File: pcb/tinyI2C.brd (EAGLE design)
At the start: 83.2 x 83.2 mm, 29 parts, among them IC1 IC_TTL_74_125, IC2 TPS73618(0.4A), U1 LPC824M201JHI33, X1 TSW-112-02-S-S, X2 TSW-106-02-S-S-RA, X3 TSW-112-02-S-S, X4 TSW-102-02-S-S, X5 TSW-102-02-S-S

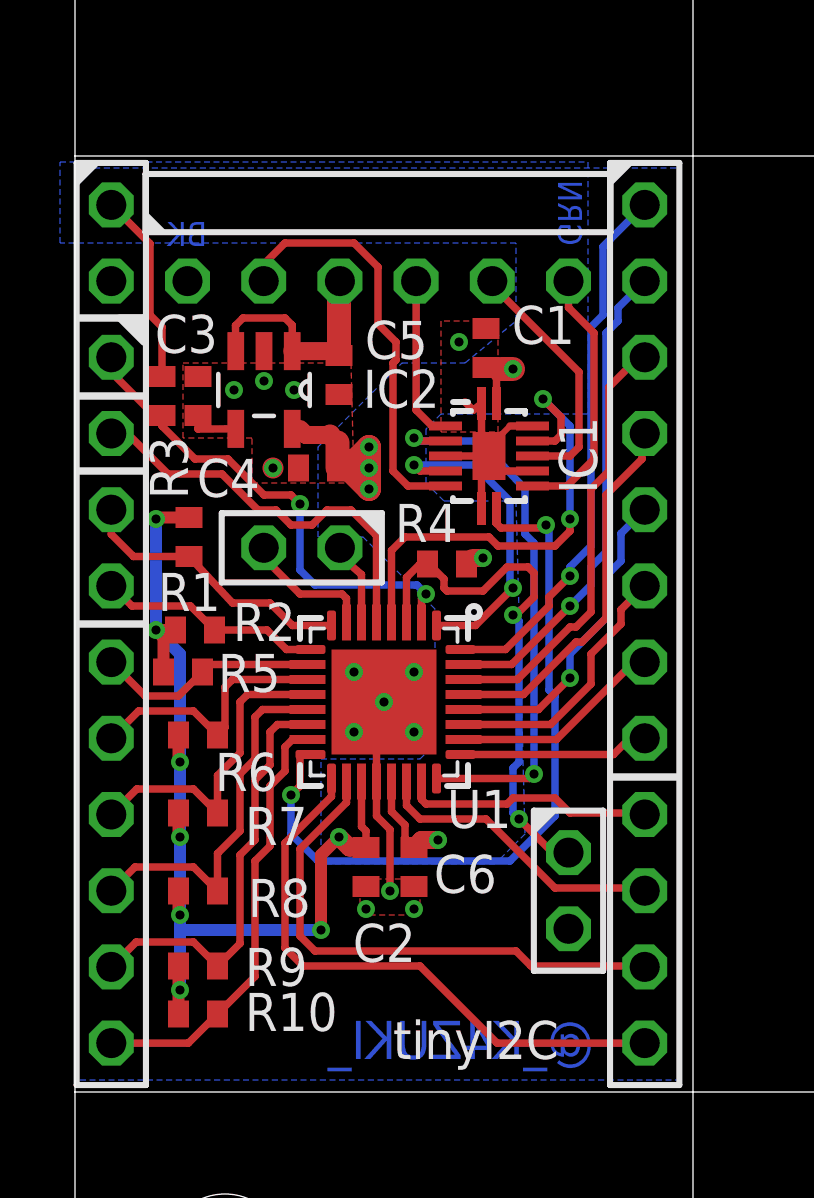
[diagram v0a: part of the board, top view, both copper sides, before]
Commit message: [ PCB ] trace change and panelize
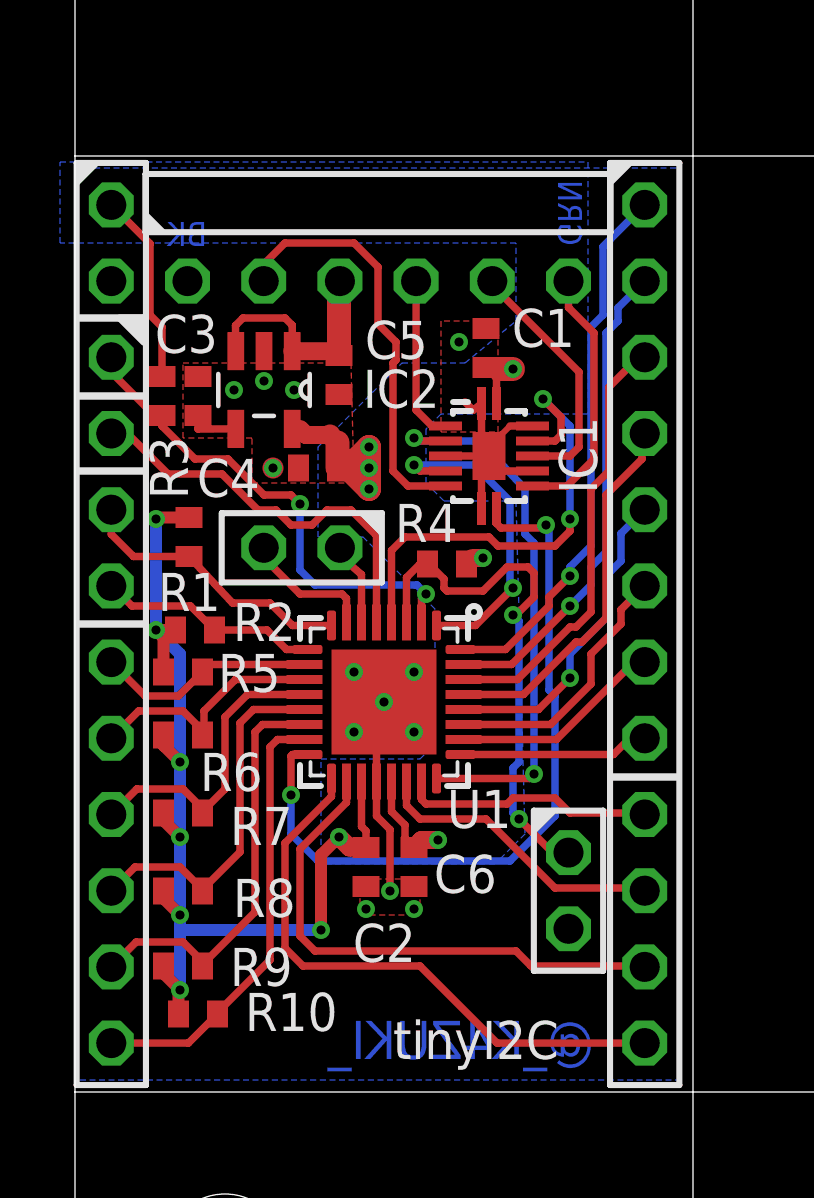
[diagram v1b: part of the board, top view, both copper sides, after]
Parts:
- moved R6 0.50 mm to (3.60, 22.3)
- moved R7 0.50 mm to (3.60, 19.7)
- moved R8 0.50 mm to (3.60, 17.1)
- moved R9 0.50 mm to (3.60, 14.6)
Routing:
- net 1.8V: track 53.9 -> 54.7 mm
